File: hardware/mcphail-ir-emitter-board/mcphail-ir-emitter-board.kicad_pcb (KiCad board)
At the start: 2 copper layers, 68.6 x 12.7 mm, 11 parts, among them J1 TO MCU

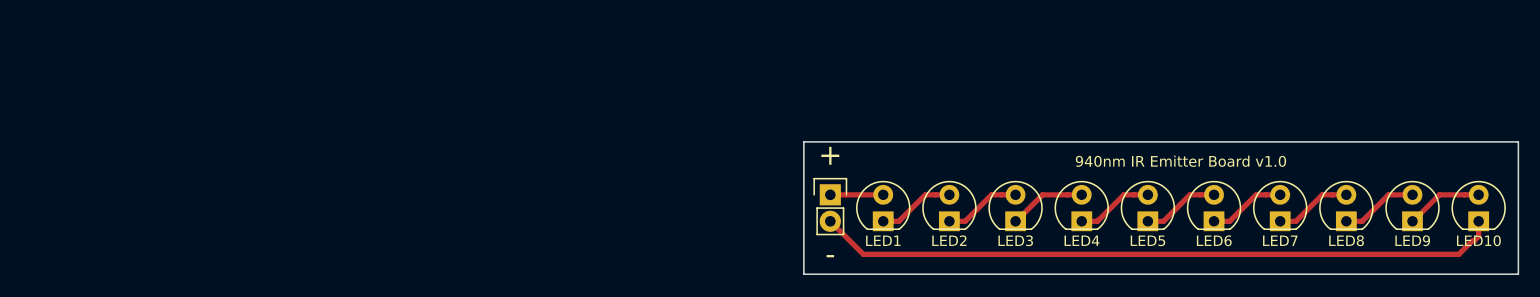
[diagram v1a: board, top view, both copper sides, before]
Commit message: Release v1.0 McPhail IR Emitter Board
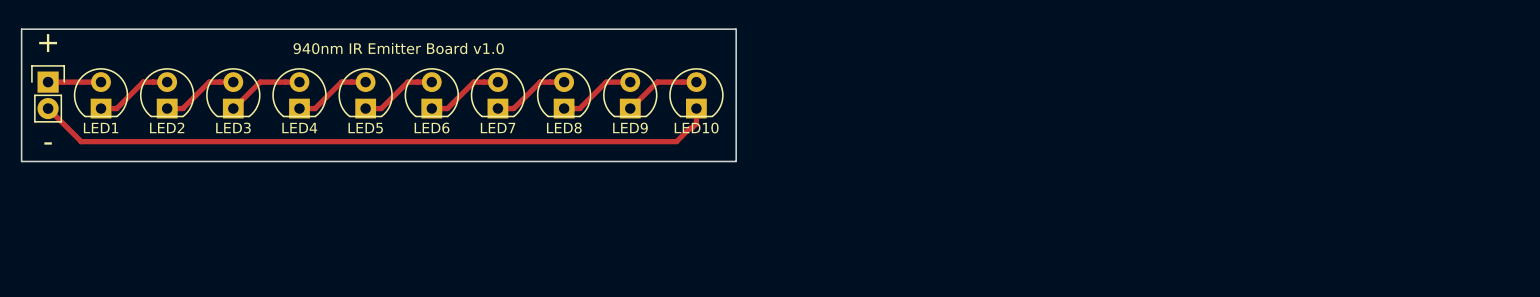
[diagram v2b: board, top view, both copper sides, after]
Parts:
- moved J1 75.9 mm to (29.1, 70.5)
- moved LED1 75.9 mm to (34.1, 73.0)
- moved LED10 75.9 mm to (91.3, 73.0)
- moved LED3 75.9 mm to (46.8, 73.0)
- moved LED4 75.9 mm to (53.2, 73.0)
- moved LED5 75.9 mm to (59.5, 73.0)
- moved LED9 75.9 mm to (84.9, 73.0)
- moved LED2 75.9 mm to (40.5, 73.0)
- moved LED6 75.9 mm to (65.9, 73.0)
- moved LED7 75.9 mm to (72.2, 73.0)
- moved LED8 75.9 mm to (78.6, 73.0)
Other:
- board text added: "FABRICATION NOTES 1. THIS IS A 2 LAYER BOARD. 2. EXTERNAL LAYERS SHALL HAVE 1 OZ COPPER. 3. MATERIAL: FR4 AND 0.062 INCH +/- 10% THICK. 4. BOARDS SHALL BE ROHS COMPLIANT. 5. MANUFACTURE IN ACCORDANCE WITH IPC-6012 CLASS 2 6. MASK: BOTH SIDES OF THE BOARD SHALL HAVE SOLDER MASK (ANY COLOR) OVER BARE COPPER. 7. SILK: BOTH SIDES OF THE BOARD SHALL HAVE WHITE SILKSCREEN. DO NOT PLACE SILK OVER BARE C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"
